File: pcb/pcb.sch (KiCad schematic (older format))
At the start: 34 parts, among them J1 Conn_02x08_Odd_Even, J2 B2B-PH-K-S_LF__SN_, Q1 MMUN2211LT1G, SW1 SW_SPST, U1 TPS61090, U2 MCP73871-1AA, X1 USB_C

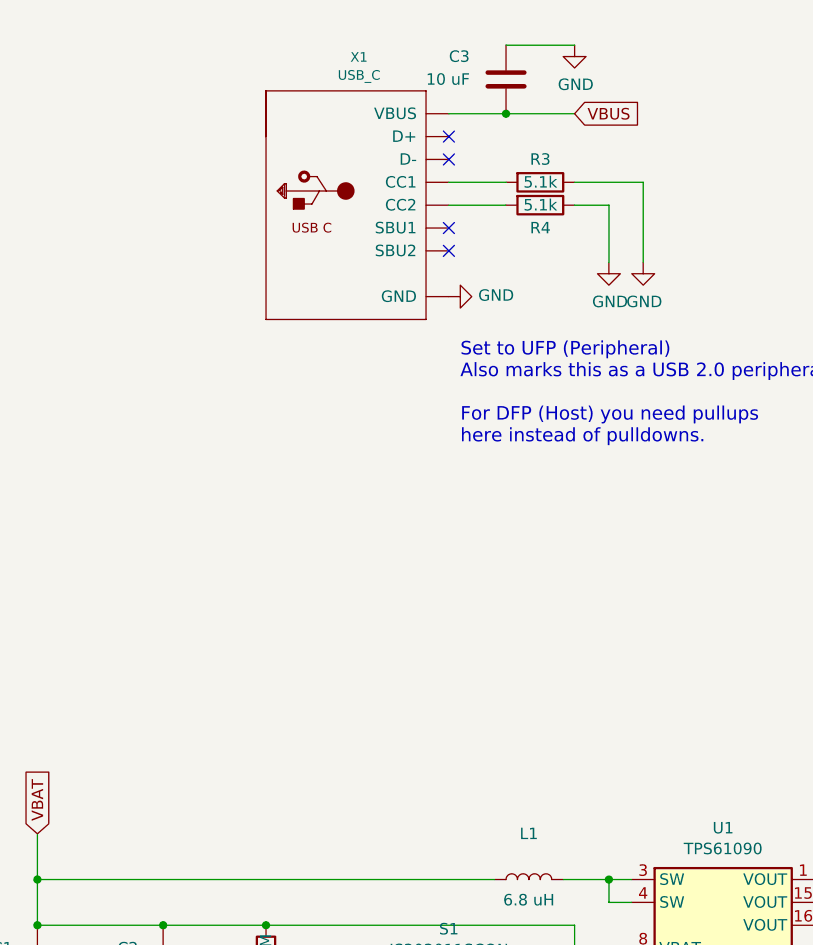
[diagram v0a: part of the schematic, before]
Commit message: pcb is compiling again
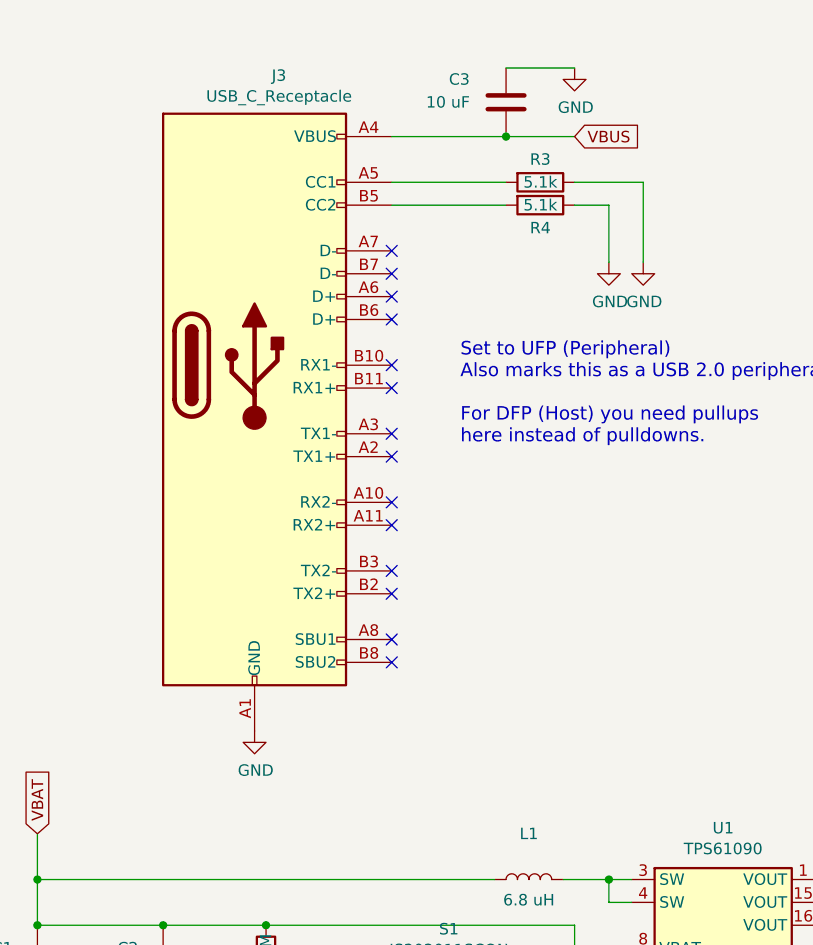
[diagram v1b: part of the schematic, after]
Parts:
- removed X1: USB_C, digikey-footprints:USB-C_Female_E8124-015-01, symbol pcb-rescue:USB_C-lipousbc-eagle-import
- added J3: USB_C_Receptacle, digikey-footprints:USB-C_Female_E8124-015-01, symbol pcb-copy:USB_C_Receptacle
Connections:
- net GND: now also J3.A1 (GND), J3.A12 (GND), J3.B1 (GND), J3.B12 (GND)
- net VBUS: now also J3.A4 (VBUS), J3.A9 (VBUS), J3.B4 (VBUS), J3.B9 (VBUS)
- net at R3.2: now also J3.A5 (CC1)
- net at R4.2: now also J3.B5 (CC2)
- no-connect marks 9 -> 19
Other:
- moved on the sheet: C3
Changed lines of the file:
@@
 	1    0    0    -1
 $EndComp
-Text GLabel 4800 3450 2    50   Input ~ 0
+Text GLabel 4800 3550 2    50   Input ~ 0
 VBUS
 Wire Wire Line
-	4500 3150 4800 3150
+	4500 3250 4800 3250
 $Comp
 L Device:R R3
@@
 $EndComp
 Wire Wire Line
-	4250 3750 4500 3750
-Wire Wire Line
-	4250 3850 4500 3850
-Wire Wire Line
 	4800 3750 5100 3750
 Wire Wire Line
@@
 L power:GND #PWR0103
 U 1 1 60123484
-P 4800 3150
-F 0 "#PWR0103" H 4800 2900 50  0001 C CNN
-F 1 "GND" H 4805 2977 50  0000 C CNN
-F 2 "" H 4800 3150 50  0001 C CNN
-F 3 "" H 4800 3150 50  0001 C CNN
-	1    4800 3150
-	1    0    0    -1
-$EndComp
-Wire Wire Line
-	4250 3450 4500 3450
+P 4800 3250
+F 0 "#PWR0103" H 4800 3000 50  0001 C CNN
+F 1 "GND" H 4805 3077 50  0000 C CNN
+F 2 "" H 4800 3250 50  0001 C CNN
+F 3 "" H 4800 3250 50  0001 C CNN
+	1    4800 3250
+	1    0    0    -1
+$EndComp
 $Comp
 L Device:C C3
 U 1 1 6012A09C
-P 4500 3300
-F 0 "C3" H 4250 3400 50  0000 L CNN
-F 1 "10 uF" H 4150 3300 50  0000 L CNN
-F 2 "Capacitor_SMD:C_0805_2012Metric" H 4538 3150 50  0001 C CNN
-F 3 "~" H 4500 3300 50  0001 C CNN
-	1    4500 3300
-	1    0    0    -1
-$EndComp
-Connection ~ 4500 3450
-Wire Wire Line
-	4500 3450 4800 3450
+P 4500 3400
+F 0 "C3" H 4250 3500 50  0000 L CNN
+F 1 "10 uF" H 4150 3400 50  0000 L CNN
+F 2 "Capacitor_SMD:C_0805_2012Metric" H 4538 3250 50  0001 C CNN
+F 3 "~" H 4500 3400 50  0001 C CNN
+	1    4500 3400
+	1    0    0    -1
+$EndComp
+Connection ~ 4500 3550
+Wire Wire Line
+	4500 3550 4800 3550
 Text Notes 4300 4900 0    59   ~ 0
 Set to UFP (Peripheral)\nAlso marks this as a USB 2.0 peripheral device\n\nFor DFP (Host) you need pullups\nhere instead of pulldowns.
@@
 F 3 "" H 11800 8250 50  0001 C CNN
 	1    11800 8250
-	1    0    0    -1
-$EndComp
-$Comp
-L power:GND #PWR0110
-U 1 1 604095B5
-P 4250 4250
-F 0 "#PWR0110" H 4250 4000 50  0001 C CNN
-F 1 "GND" V 4255 4122 50  0000 R CNN
-F 2 "" H 4250 4250 50  0001 C CNN
-F 3 "" H 4250 4250 50  0001 C CNN
-	1    4250 4250
-	0    -1   -1   0
-$EndComp
-NoConn ~ 4250 4050
-NoConn ~ 4250 3950
-NoConn ~ 4250 3650
-NoConn ~ 4250 3550
-$Comp
-L pcb-rescue:USB_C-lipousbc-eagle-import X1
-U 1 1 60044940
-P 3850 3850
-F 0 "X1" H 3857 4497 42  0000 C CNN
-F 1 "USB_C" H 3857 4418 42  0000 C CNN
-F 2 "digikey-footprints:USB-C_Female_E8124-015-01" H 3850 3850 50  0001 C CNN
-F 3 "" H 3850 3850 50  0001 C CNN
-	1    3850 3850
 	1    0    0    -1
 $EndComp
@@
 	1    0    0    -1
 $EndComp
+Wire Wire Line
+	4000 3550 4500 3550
+Wire Wire Line
+	4000 3750 4500 3750
+Wire Wire Line
+	4000 3850 4500 3850
+$Comp
+L power:GND #PWR0110
+U 1 1 5F427914
+P 3400 6150
+F 0 "#PWR0110" H 3400 5900 50  0001 C CNN
+F 1 "GND" H 3405 5977 50  0000 C CNN
+F 2 "" H 3400 6150 50  0001 C CNN
+F 3 "" H 3400 6150 50  0001 C CNN
+	1    3400 6150
+	1    0    0    -1
+$EndComp
+NoConn ~ 4000 4050
+NoConn ~ 4000 4150
+NoConn ~ 4000 4250
+NoConn ~ 4000 4350
+NoConn ~ 4000 4550
+NoConn ~ 4000 4650
+NoConn ~ 4000 4850
+NoConn ~ 4000 4950
+NoConn ~ 4000 5150
+NoConn ~ 4000 5250
+NoConn ~ 4000 5450
+NoConn ~ 4000 5550
+NoConn ~ 4000 5750
+NoConn ~ 4000 5850
+$Comp
+L pcb-copy:USB_C_Receptacle J3
+U 1 1 5F483AEA
+P 3400 4550
+F 0 "J3" H 3507 5817 50  0000 C CNN
+F 1 "USB_C_Receptacle" H 3507 5726 50  0000 C CNN
+F 2 "digikey-footprints:USB-C_Female_E8124-015-01" H 3550 4550 50  0001 C CNN
+F 3 "https://www.usb.org/sites/default/files/documents/usb_type-c.zip" H 3550 4550 50  0001 C CNN
+	1    3400 4550
+	1    0    0    -1
+$EndComp

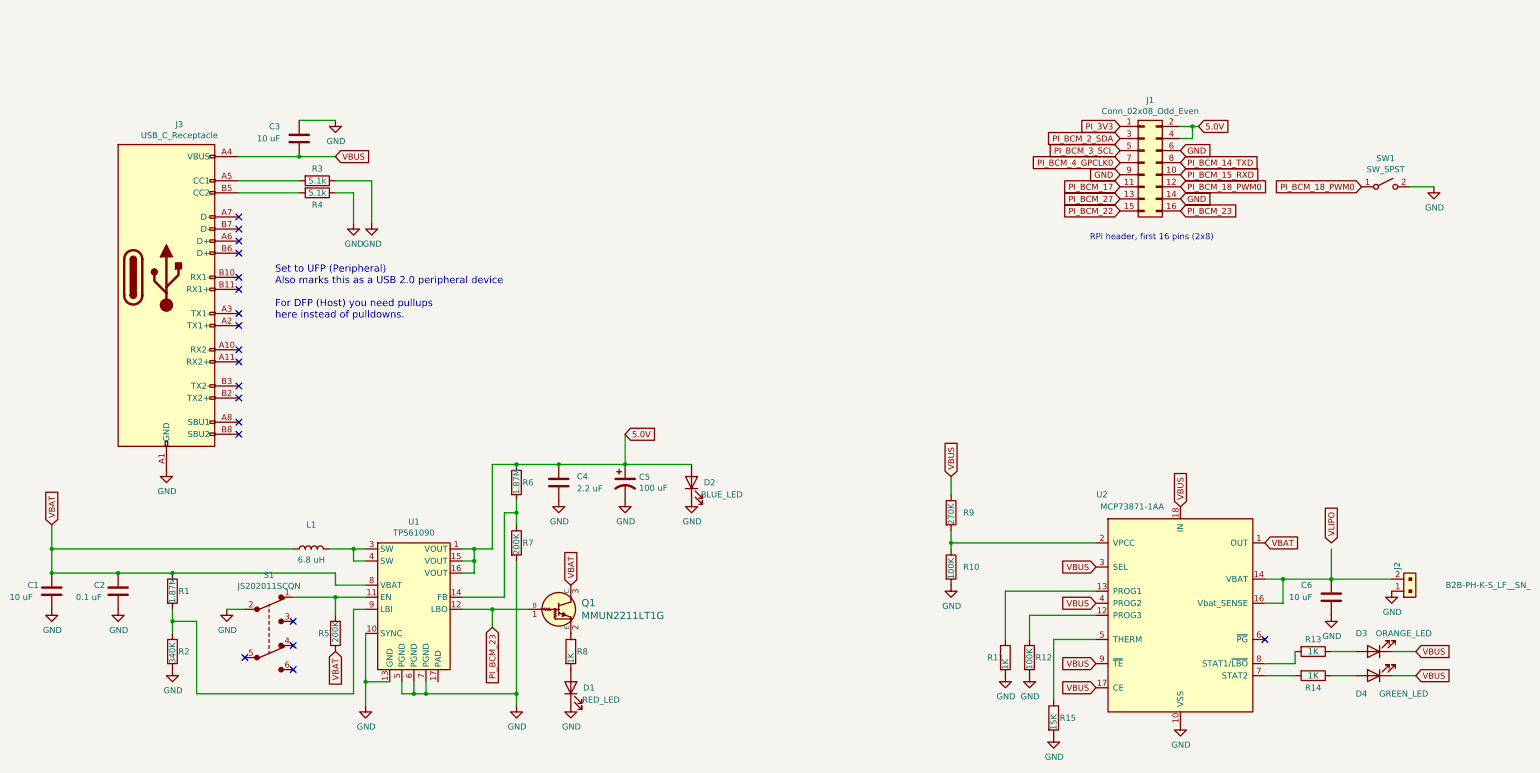
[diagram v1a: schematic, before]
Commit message: in work, PCB layup
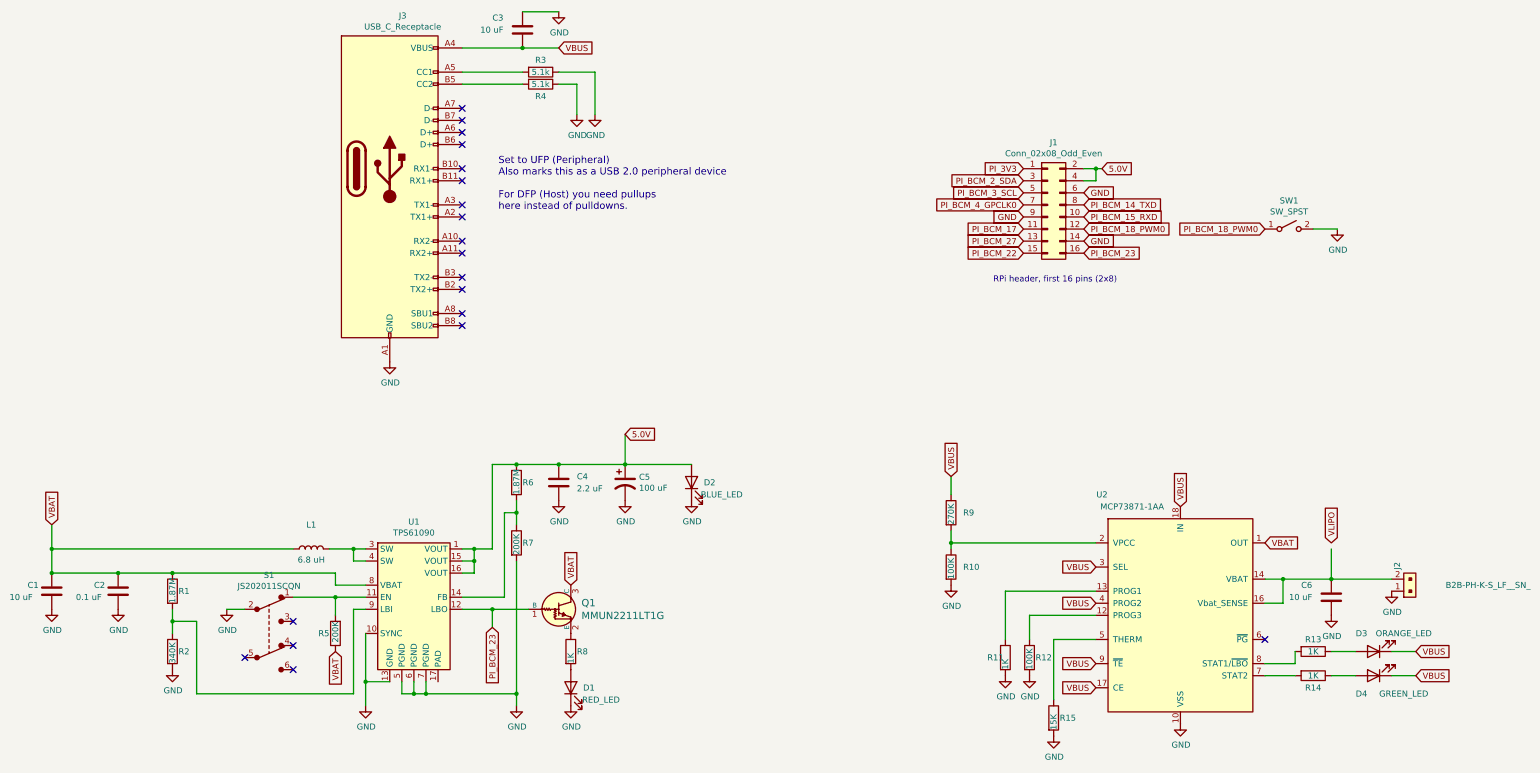
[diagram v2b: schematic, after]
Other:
- moved on the sheet: C3, J1, J3, R3, R4, SW1
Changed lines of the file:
@@
 	0    -1   -1   0
 $EndComp
-Text Notes 11050 4250 0    50   ~ 0
+Text Notes 10250 4600 0    50   ~ 0
 RPi header, first 16 pins (2x8)
 $Comp
 L Connector_Generic:Conn_02x08_Odd_Even J1
 U 1 1 5F8C44B2
-P 11500 3600
-F 0 "J1" H 11550 4117 50  0000 C CNN
-F 1 "Conn_02x08_Odd_Even" H 11550 4026 50  0000 C CNN
-F 2 "Connector_PinHeader_2.54mm:PinHeader_2x08_P2.54mm_Vertical" H 11500 3600 50  0001 C CNN
-F 3 "~" H 11500 3600 50  0001 C CNN
-	1    11500 3600
-	1    0    0    -1
-$EndComp
-Text GLabel 4800 3550 2    50   Input ~ 0
+P 10700 3950
+F 0 "J1" H 10750 4467 50  0000 C CNN
+F 1 "Conn_02x08_Odd_Even" H 10750 4376 50  0000 C CNN
+F 2 "Connector_PinHeader_2.54mm:PinHeader_2x08_P2.54mm_Vertical" H 10700 3950 50  0001 C CNN
+F 3 "~" H 10700 3950 50  0001 C CNN
+	1    10700 3950
+	1    0    0    -1
+$EndComp
+Text GLabel 6650 2650 2    50   Input ~ 0
 VBUS
 Wire Wire Line
-	4500 3250 4800 3250
+	6350 2350 6650 2350
 $Comp
 L Device:R R3
 U 1 1 600F42D8
-P 4650 3750
-F 0 "R3" V 4550 3750 50  0000 C CNN
-F 1 "5.1k" V 4650 3750 50  0000 C CNN
-F 2 "Resistor_SMD:R_0402_1005Metric" V 4580 3750 50  0001 C CNN
-F 3 "https://www.digikey.com/product-detail/en/yageo/RC0402FR-075K1L/311-5-10KLRCT-ND/729571" H 4650 3750 50  0001 C CNN
-	1    4650 3750
+P 6500 2850
+F 0 "R3" V 6400 2850 50  0000 C CNN
+F 1 "5.1k" V 6500 2850 50  0000 C CNN
+F 2 "Resistor_SMD:R_0402_1005Metric" V 6430 2850 50  0001 C CNN
+F 3 "https://www.digikey.com/product-detail/en/yageo/RC0402FR-075K1L/311-5-10KLRCT-ND/729571" H 6500 2850 50  0001 C CNN
+	1    6500 2850
 	0    1    1    0
 $EndComp
@@
 L Device:R R4
 U 1 1 600F482B
-P 4650 3850
-F 0 "R4" V 4750 3850 50  0000 C CNN
-F 1 "5.1k" V 4650 3850 50  0000 C CNN
-F 2 "Resistor_SMD:R_0402_1005Metric" V 4580 3850 50  0001 C CNN
-F 3 "~" H 4650 3850 50  0001 C CNN
-	1    4650 3850
+P 6500 2950
+F 0 "R4" V 6600 2950 50  0000 C CNN
+F 1 "5.1k" V 6500 2950 50  0000 C CNN
+F 2 "Resistor_SMD:R_0402_1005Metric" V 6430 2950 50  0001 C CNN
+F 3 "~" H 6500 2950 50  0001 C CNN
+	1    6500 2950
 	0    1    1    0
 $EndComp
 Wire Wire Line
-	4800 3750 5100 3750
-Wire Wire Line
-	5100 3750 5100 4100
-Wire Wire Line
-	4800 3850 4950 3850
-Wire Wire Line
-	4950 3850 4950 4100
+	6650 2850 6950 2850
+Wire Wire Line
+	6950 2850 6950 3200
+Wire Wire Line
+	6650 2950 6800 2950
+Wire Wire Line
+	6800 2950 6800 3200
 $Comp
 L power:GND #PWR0101
 U 1 1 60122058
-P 4950 4100
-F 0 "#PWR0101" H 4950 3850 50  0001 C CNN
-F 1 "GND" H 4955 3927 50  0000 C CNN
-F 2 "" H 4950 4100 50  0001 C CNN
-F 3 "" H 4950 4100 50  0001 C CNN
-	1    4950 4100
+P 6800 3200
+F 0 "#PWR0101" H 6800 2950 50  0001 C CNN
+F 1 "GND" H 6805 3027 50  0000 C CNN
+F 2 "" H 6800 3200 50  0001 C CNN
+F 3 "" H 6800 3200 50  0001 C CNN
+	1    6800 3200
 	1    0    0    -1
 $EndComp
@@
 L power:GND #PWR0102
 U 1 1 60123124
-P 5100 4100
-F 0 "#PWR0102" H 5100 3850 50  0001 C CNN
-F 1 "GND" H 5105 3927 50  0000 C CNN
-F 2 "" H 5100 4100 50  0001 C CNN
-F 3 "" H 5100 4100 50  0001 C CNN
-	1    5100 4100
+P 6950 3200
+F 0 "#PWR0102" H 6950 2950 50  0001 C CNN
+F 1 "GND" H 6955 3027 50  0000 C CNN
+F 2 "" H 6950 3200 50  0001 C CNN
+F 3 "" H 6950 3200 50  0001 C CNN
+	1    6950 3200
 	1    0    0    -1
 $EndComp
@@
 L power:GND #PWR0103
 U 1 1 60123484
-P 4800 3250
-F 0 "#PWR0103" H 4800 3000 50  0001 C CNN
-F 1 "GND" H 4805 3077 50  0000 C CNN
-F 2 "" H 4800 3250 50  0001 C CNN
-F 3 "" H 4800 3250 50  0001 C CNN
-	1    4800 3250
+P 6650 2350
+F 0 "#PWR0103" H 6650 2100 50  0001 C CNN
+F 1 "GND" H 6655 2177 50  0000 C CNN
+F 2 "" H 6650 2350 50  0001 C CNN
+F 3 "" H 6650 2350 50  0001 C CNN
+	1    6650 2350
 	1    0    0    -1
 $EndComp
@@
 L Device:C C3
 U 1 1 6012A09C
-P 4500 3400
-F 0 "C3" H 4250 3500 50  0000 L CNN
-F 1 "10 uF" H 4150 3400 50  0000 L CNN
-F 2 "Capacitor_SMD:C_0805_2012Metric" H 4538 3250 50  0001 C CNN
-F 3 "~" H 4500 3400 50  0001 C CNN
-	1    4500 3400
-	1    0    0    -1
-$EndComp
-Connection ~ 4500 3550
-Wire Wire Line
-	4500 3550 4800 3550
-Text Notes 4300 4900 0    59   ~ 0
+P 6350 2500
+F 0 "C3" H 6100 2600 50  0000 L CNN
+F 1 "10 uF" H 6000 2500 50  0000 L CNN
+F 2 "Capacitor_SMD:C_0805_2012Metric" H 6388 2350 50  0001 C CNN
+F 3 "~" H 6350 2500 50  0001 C CNN
+	1    6350 2500
+	1    0    0    -1
+$EndComp
+Connection ~ 6350 2650
+Wire Wire Line
+	6350 2650 6650 2650
+Text Notes 6150 4000 0    59   ~ 0
 Set to UFP (Peripheral)\nAlso marks this as a USB 2.0 peripheral device\n\nFor DFP (Host) you need pullups\nhere instead of pulldowns.
 Text GLabel 9900 6200 1    50   Input ~ 0
@@
 Text GLabel 11800 6450 1    50   Input ~ 0
 VBUS
-Text GLabel 11800 3500 2    50   Input ~ 0
+Text GLabel 11000 3850 2    50   Input ~ 0
 GND
-Text GLabel 11800 3600 2    50   Input ~ 0
+Text GLabel 11000 3950 2    50   Input ~ 0
 PI_BCM_14_TXD
-Text GLabel 11800 3700 2    50   Input ~ 0
+Text GLabel 11000 4050 2    50   Input ~ 0
 PI_BCM_15_RXD
-Text GLabel 11800 3800 2    50   Input ~ 0
+Text GLabel 11000 4150 2    50   Input ~ 0
 PI_BCM_18_PWM0
-Text GLabel 11800 3900 2    50   Input ~ 0
+Text GLabel 11000 4250 2    50   Input ~ 0
 GND
-Text GLabel 11800 4000 2    50   Input ~ 0
+Text GLabel 11000 4350 2    50   Input ~ 0
 PI_BCM_23
-Text GLabel 11300 3300 0    50   Input ~ 0
+Text GLabel 10500 3650 0    50   Input ~ 0
 PI_3V3
-Text GLabel 11300 3400 0    50   Input ~ 0
+Text GLabel 10500 3750 0    50   Input ~ 0
 PI_BCM_2_SDA
-Text GLabel 11300 3500 0    50   Input ~ 0
+Text GLabel 10500 3850 0    50   Input ~ 0
 PI_BCM_3_SCL
-Text GLabel 11300 3600 0    50   Input ~ 0
+Text GLabel 10500 3950 0    50   Input ~ 0
 PI_BCM_4_GPCLK0
-Text GLabel 11300 3700 0    50   Input ~ 0
+Text GLabel 10500 4050 0    50   Input ~ 0
 GND
-Text GLabel 11300 3800 0    50   Input ~ 0
+Text GLabel 10500 4150 0    50   Input ~ 0
 PI_BCM_17
-Text GLabel 11300 3900 0    50   Input ~ 0
+Text GLabel 10500 4250 0    50   Input ~ 0
 PI_BCM_27
-Text GLabel 11300 4000 0    50   Input ~ 0
+Text GLabel 10500 4350 0    50   Input ~ 0
 PI_BCM_22
 $Comp
@@
 Wire Wire Line
 	13050 7050 13550 7050
-Text GLabel 11950 3300 2    50   Input ~ 0
+Text GLabel 11150 3650 2    50   Input ~ 0
 5.0V
 Wire Wire Line
-	11800 3300 11900 3300
-Wire Wire Line
-	11800 3400 11900 3400
-Wire Wire Line
-	11900 3400 11900 3300
-Connection ~ 11900 3300
-Wire Wire Line
-	11900 3300 11950 3300
+	11000 3650 11100 3650
+Wire Wire Line
+	11000 3750 11100 3750
+Wire Wire Line
+	11100 3750 11100 3650
+Connection ~ 11100 3650
+Wire Wire Line
+	11100 3650 11150 3650
 $Comp
 L dk_Transistors-Bipolar-BJT-Single-Pre-Biased:MMUN2211LT1G Q1
@@
 L power:GND #PWR0113
 U 1 1 5F5EA593
-P 13900 3800
-F 0 "#PWR0113" H 13900 3550 50  0001 C CNN
-F 1 "GND" H 13905 3627 50  0000 C CNN
-F 2 "" H 13900 3800 50  0001 C CNN
-F 3 "" H 13900 3800 50  0001 C CNN
-	1    13900 3800
-	1    0    0    -1
-$EndComp
-Wire Wire Line
-	13700 3800 13900 3800
-Text GLabel 13300 3800 0    50   Input ~ 0
+P 13100 4150
+F 0 "#PWR0113" H 13100 3900 50  0001 C CNN
+F 1 "GND" H 13105 3977 50  0000 C CNN
+F 2 "" H 13100 4150 50  0001 C CNN
+F 3 "" H 13100 4150 50  0001 C CNN
+	1    13100 4150
+	1    0    0    -1
+$EndComp
+Wire Wire Line
+	12900 4150 13100 4150
+Text GLabel 12500 4150 0    50   Input ~ 0
 PI_BCM_18_PWM0
 Text GLabel 6750 7100 1    50   Input ~ 0
@@
 L Switch:SW_SPST SW1
 U 1 1 5F5697F6
-P 13500 3800
-F 0 "SW1" H 13500 4035 50  0000 C CNN
-F 1 "SW_SPST" H 13500 3944 50  0000 C CNN
-F 2 "tinycam:FP11SPA1B1TP00" H 13500 3800 50  0001 C CNN
-F 3 "https://www.digikey.com/product-detail/en/judco-manufacturing-inc/50-0014-00/518PB-ND/307996" H 13500 3800 50  0001 C CNN
-	1    13500 3800
-	1    0    0    -1
-$EndComp
-Wire Wire Line
-	4000 3550 4500 3550
-Wire Wire Line
-	4000 3750 4500 3750
-Wire Wire Line
-	4000 3850 4500 3850
+P 12700 4150
+F 0 "SW1" H 12700 4385 50  0000 C CNN
+F 1 "SW_SPST" H 12700 4294 50  0000 C CNN
+F 2 "tinycam:FP11SPA1B1TP00" H 12700 4150 50  0001 C CNN
+F 3 "https://www.digikey.com/product-detail/en/judco-manufacturing-inc/50-0014-00/518PB-ND/307996" H 12700 4150 50  0001 C CNN
+	1    12700 4150
+	1    0    0    -1
+$EndComp
+Wire Wire Line
+	5850 2650 6350 2650
+Wire Wire Line
+	5850 2850 6350 2850
+Wire Wire Line
+	5850 2950 6350 2950
 $Comp
 L power:GND #PWR0110
 U 1 1 5F427914
-P 3400 6150
-F 0 "#PWR0110" H 3400 5900 50  0001 C CNN
-F 1 "GND" H 3405 5977 50  0000 C CNN
-F 2 "" H 3400 6150 50  0001 C CNN
-F 3 "" H 3400 6150 50  0001 C CNN
-	1    3400 6150
-	1    0    0    -1
-$EndComp
-NoConn ~ 4000 4050
-NoConn ~ 4000 4150
-NoConn ~ 4000 4250
-NoConn ~ 4000 4350
-NoConn ~ 4000 4550
-NoConn ~ 4000 4650
-NoConn ~ 4000 4850
-NoConn ~ 4000 4950
-NoConn ~ 4000 5150
-NoConn ~ 4000 5250
-NoConn ~ 4000 5450
-NoConn ~ 4000 5550
-NoConn ~ 4000 5750
-NoConn ~ 4000 5850
+P 5250 5250
+F 0 "#PWR0110" H 5250 5000 50  0001 C CNN
+F 1 "GND" H 5255 5077 50  0000 C CNN
+F 2 "" H 5250 5250 50  0001 C CNN
+F 3 "" H 5250 5250 50  0001 C CNN
+	1    5250 5250
+	1    0    0    -1
+$EndComp
+NoConn ~ 5850 3150
+NoConn ~ 5850 3250
+NoConn ~ 5850 3350
+NoConn ~ 5850 3450
+NoConn ~ 5850 3650
+NoConn ~ 5850 3750
+NoConn ~ 5850 3950
+NoConn ~ 5850 4050
+NoConn ~ 5850 4250
+NoConn ~ 5850 4350
+NoConn ~ 5850 4550
+NoConn ~ 5850 4650
+NoConn ~ 5850 4850
+NoConn ~ 5850 4950
 $Comp
 L pcb-copy:USB_C_Receptacle J3
 U 1 1 5F483AEA
-P 3400 4550
-F 0 "J3" H 3507 5817 50  0000 C CNN
-F 1 "USB_C_Receptacle" H 3507 5726 50  0000 C CNN
-F 2 "digikey-footprints:USB-C_Female_E8124-015-01" H 3550 4550 50  0001 C CNN
-F 3 "https://www.usb.org/sites/default/files/documents/usb_type-c.zip" H 3550 4550 50  0001 C CNN
-	1    3400 4550
-	1    0    0    -1
-$EndComp
+P 5250 3650
+F 0 "J3" H 5357 4917 50  0000 C CNN
+F 1 "USB_C_Receptacle" H 5357 4826 50  0000 C CNN
+F 2 "digikey-footprints:USB-C_Female_E8124-015-01" H 5400 3650 50  0001 C CNN
+F 3 "https://www.usb.org/sites/default/files/documents/usb_type-c.zip" H 5400 3650 50  0001 C CNN
+	1    5250 3650
+	1    0    0    -1
+$EndComp
